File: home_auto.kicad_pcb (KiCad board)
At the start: 2 copper layers, 162 parts, among them J1 Conn_01x08_Pin, J10 Screw_Terminal_01x02, J11 Screw_Terminal_01x02, J12 Screw_Terminal_01x02, J13 Screw_Terminal_01x02, J14 Screw_Terminal_01x02, J15 Screw_Terminal_01x02, J16 Screw_Terminal_01x02, J17 Screw_Terminal_01x02, J18 Screw_Terminal_01x02, J19 Screw_Terminal_01x02, J2 Screw_Terminal_01x02, J20 Screw_Terminal_01x02, J21 Screw_Terminal_01x02, J22 Screw_Terminal_01x02, J23 Screw_Terminal_01x02, J24 Screw_Terminal_01x02, J25 Screw_Terminal_01x02, J26 Conn_01x02_Pin, J27 Conn_01x04_Pin, J28 Conn_01x02_Pin, J29 TC0203620000G, J3 Screw_Terminal_01x02, J4 Conn_02x10_Top_Bottom, J5 Conn_02x10_Top_Bottom, J6 Screw_Terminal_01x02, J7 Screw_Terminal_01x02, J8 Screw_Terminal_01x02, J9 Screw_Terminal_01x02, K1 G5NB-1A4_DC5, K10 G5NB-1A4_DC5, K11 G5NB-1A4_DC5, K12 G5NB-1A4_DC5, K13 G5NB-1A4_DC5, K14 G5NB-1A4_DC5, K15 G5NB-1A4_DC5, K16 G5NB-1A4_DC5, K17 G5NB-1A4_DC5, K18 G5NB-1A4_DC5, K19 G5NB-1A4_DC5, K2 G5NB-1A4_DC5, K20 G5NB-1A4_DC5, K21 G5NB-1A4_DC5, K22 G5NB-1A4_DC5, K23 G5NB-1A4_DC5, K24 G5NB-1A4_DC5, K25 G5NB-1A4_DC5, K26 G5NB-1A4_DC5, K27 G5NB-1A4_DC5, K28 G5NB-1A4_DC5, K3 G5NB-1A4_DC5, K4 G5NB-1A4_DC5, K5 G5NB-1A4_DC5, K6 G5NB-1A4_DC5, K7 G5NB-1A4_DC5, K8 G5NB-1A4_DC5, K9 G5NB-1A4_DC5, Q1 BC849, Q10 BC849, Q11 BC849, Q12 BC849, Q13 BC849, Q14 BC849, Q15 BC849, Q16 BC849, Q17 BC849, Q18 BC849, Q19 BC849, Q2 BC849, Q20 BC849, Q21 BC849, Q22 BC849, Q23 BC849, Q24 BC849, Q25 BC849, Q26 BC849, Q27 BC849, Q28 BC849, Q3 BC849, Q4 BC849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

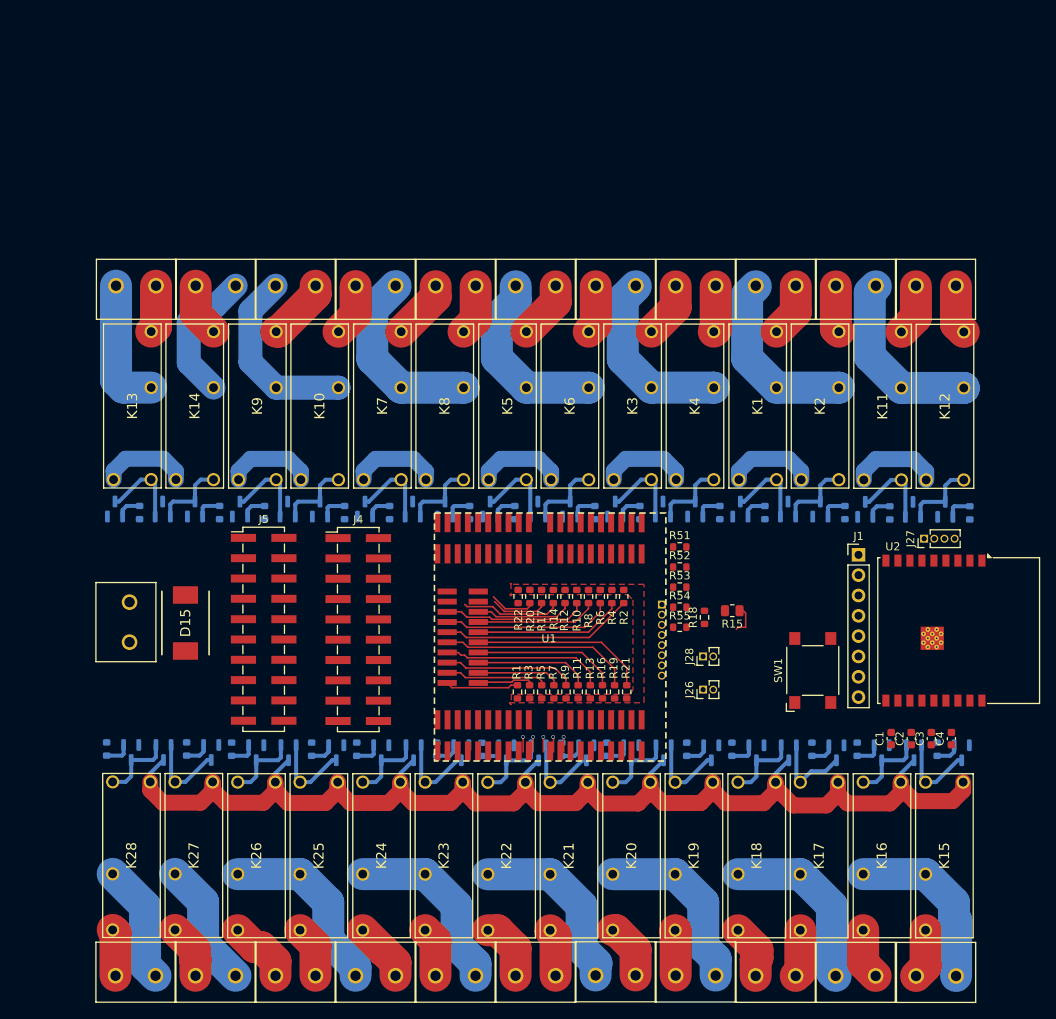
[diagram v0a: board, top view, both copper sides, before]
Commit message: filse fo JCL pcb generated
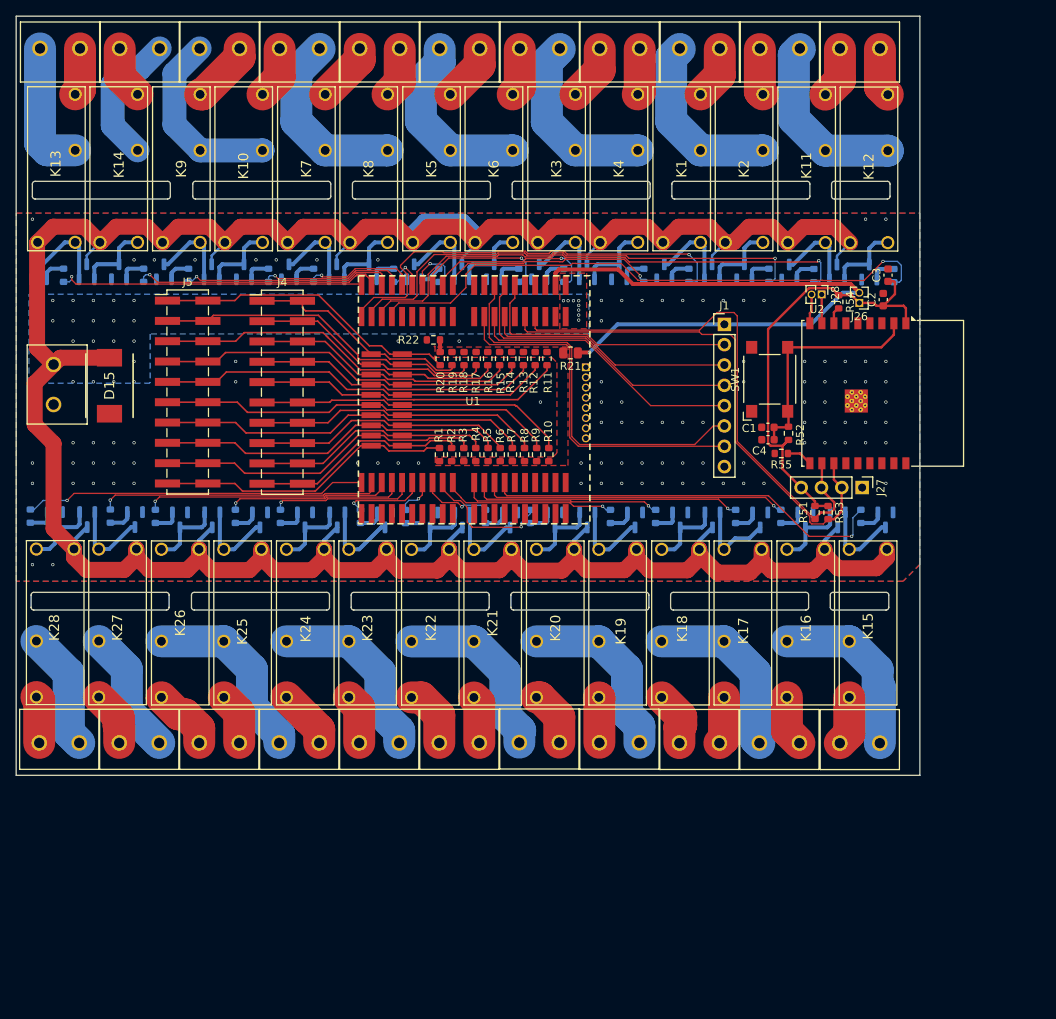
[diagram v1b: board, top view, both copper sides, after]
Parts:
- J27: footprint Connector_PinHeader_1.27mm:PinHeader_1x04_P1.27mm_Vertical -> Connector_PinHeader_2.54mm:PinHeader_1x04_P2.54mm_Vertical
- R15: value 0R -> 4K7; footprint Resistor_SMD:R_0805_2012Metric -> Resistor_SMD:R_0603_1608Metric
- R18: value 0R -> 4K7
- R21: value 4K7 -> 0R; footprint Resistor_SMD:R_0603_1608Metric -> Resistor_SMD:R_0805_2012Metric
- R22: value 4K7 -> 0R
- moved C3 58.2 mm to (250.6, 81.7)
- moved C2 55.0 mm to (250.0, 84.8)
- moved J26 52.1 mm to (247.0, 85.2), turned to 180 degrees
- moved J28 47.6 mm to (242.3, 84.1), turned to -90 degrees
- moved R19 46.3 mm to (196.1, 92.1), turned to 90 degrees
- moved R18 44.2 mm to (197.6, 92.1)
- moved R16 44.1 mm to (200.5, 92.1), turned to 90 degrees
- moved C4 43.8 mm to (235.6, 102.3), turned to 180 degrees
- moved R54 43.0 mm to (244.4, 85.0), turned to -90 degrees
- moved R21 42.9 mm to (210.9, 91.4), turned to 180 degrees
- moved R15 42.9 mm to (202.0, 92.1), turned to 90 degrees
- moved R13 42.5 mm to (205.0, 92.1), turned to 90 degrees
- moved C1 41.9 mm to (235.6, 100.7), turned to 180 degrees
- moved R11 41.8 mm to (207.9, 92.1), turned to 90 degrees
- moved SW1 36.8 mm to (235.8, 94.7)
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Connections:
- J4 pad 1: /sw_13 -> /sw_18
- J4 pad 10: /sw_14 -> /sw_10
- J4 pad 11: /sw_15 -> /sw_9
- J4 pad 12: /sw_15 -> /sw_9
- J4 pad 13: /sw_16 -> /sw_7
- J4 pad 14: /sw_16 -> /sw_7
- J4 pad 15: /sw_17 -> /sw_5
- J4 pad 16: /sw_17 -> /sw_5
- J4 pad 17: /sw_18 -> /sw_3
- J4 pad 18: /sw_18 -> /sw_3
- J4 pad 19: /sw_19 -> /sw_1
- J4 pad 2: /sw_13 -> /sw_18
- J4 pad 20: /sw_19 -> /sw_1
- J4 pad 3: /sw_12 -> /sw_16
- J4 pad 4: /sw_12 -> /sw_16
- J4 pad 5: /sw_11 -> /sw_14
- J4 pad 6: /sw_11 -> /sw_14
- J4 pad 7: /sw_10 -> /sw_12
- J4 pad 8: /sw_10 -> /sw_12
- J4 pad 9: /sw_14 -> /sw_10
- J5 pad 1: /sw_3 -> /sw_19
- J5 pad 10: /sw_4 -> /sw_11
- J5 pad 11: /sw_5 -> /sw_8
- J5 pad 12: /sw_5 -> /sw_8
- J5 pad 15: /sw_7 -> /sw_4
- J5 pad 16: /sw_7 -> /sw_4
- J5 pad 17: /sw_8 -> /sw_2
- J5 pad 18: /sw_8 -> /sw_2
- J5 pad 19: /sw_9 -> /sw_0
- J5 pad 2: /sw_3 -> /sw_19
- J5 pad 20: /sw_9 -> /sw_0
- J5 pad 3: /sw_2 -> /sw_17
- J5 pad 4: /sw_2 -> /sw_17
- J5 pad 5: /sw_1 -> /sw_15
- J5 pad 6: /sw_1 -> /sw_15
- J5 pad 7: /sw_0 -> /sw_13
- J5 pad 8: /sw_0 -> /sw_13
- J5 pad 9: /sw_4 -> /sw_11
- R1 pad 1: /sw_10 -> /sw_0
- R10 pad 1: /sw_4 -> /sw_9
- R11 pad 1: /sw_15 -> /sw_10
- R12 pad 1: /sw_5 -> /sw_11
- R13 pad 1: /sw_16 -> /sw_12
- R14 pad 1: /sw_6 -> /sw_13
- R15 pad 1: +3V3 -> /sw_14
- R16 pad 1: /sw_17 -> /sw_15
- R17 pad 1: /sw_7 -> /sw_16
- R18 pad 1: GND -> /sw_17
- R2 pad 1: /sw_0 -> /sw_1
- R20 pad 1: /sw_8 -> /sw_19
- R21 pad 1: /sw_19 -> +3V3
- R22 pad 1: /sw_9 -> GND
- R23 pad 2: /led_cur_lim2/UP -> /up_2
- R24 pad 2: /led_cur_lim2/DOWN -> /down_2
- R25 pad 2: /led_cur_lim3/UP -> /up_3
- R26 pad 2: /led_cur_lim3/DOWN -> /down_3
- R27 pad 2: /led_cur_lim4/UP -> /up_4
- R28 pad 2: /led_cur_lim4/DOWN -> /down_4
- R29 pad 2: /led_cur_lim5/UP -> /up_5
- R3 pad 1: /sw_11 -> /sw_2
- R30 pad 2: /led_cur_lim5/DOWN -> /down_5
- R31 pad 2: /led_cur_lim6/UP -> /up_6
- R32 pad 2: /led_cur_lim6/DOWN -> /down_6
- R33 pad 2: /led_cur_lim1/UP -> /up_1
- R34 pad 2: /led_cur_lim1/DOWN -> /down_1
- R35 pad 2: /led_cur_lim7/UP -> /up_7
- R36 pad 2: /led_cur_lim7/DOWN -> /down_7
- R37 pad 2: /led_cur_lim8/UP -> /up_8
- R38 pad 2: /led_cur_lim8/DOWN -> /down_8
- R39 pad 2: /led_cur_lim9/UP -> /up_9
- R4 pad 1: /sw_1 -> /sw_3
- R40 pad 2: /led_cur_lim9/DOWN -> /down_9
- R41 pad 2: /led_cur_lim10/UP -> /up_A
- R42 pad 2: /led_cur_lim10/DOWN -> /down_A
- R43 pad 2: /led_cur_lim11/UP -> /up_B
- R44 pad 2: /led_cur_lim11/DOWN -> /down_B
- R45 pad 2: /led_cur_lim12/UP -> /up_C
- R46 pad 2: /led_cur_lim12/DOWN -> /down_C
- R47 pad 2: /led_cur_lim13/UP -> /up_D
- R48 pad 2: /led_cur_lim13/DOWN -> /down_D
- R49 pad 2: /led_cur_lim14/UP -> /up_E
- R5 pad 1: /sw_12 -> /sw_4
- R50 pad 2: /led_cur_lim14/DOWN -> /down_E
- R6 pad 1: /sw_2 -> /sw_5
- R7 pad 1: /sw_13 -> /sw_6
- R8 pad 1: /sw_3 -> /sw_7
- R9 pad 1: /sw_14 -> /sw_8
- U1 pad B11: /RX -> /TX
- U1 pad B13: /TX -> /RX
- U1 pad C0: /UP_12 -> /up_7
- U1 pad C1: unconnected-(U1B-GPIO15-PadC1) -> /up_2
- U1 pad C10: /DOWN_14 -> /down_5
- U1 pad C12: /UP_14 -> /up_4
- U1 pad C14: /DOWN_13 -> /down_4
- U1 pad C16: /UP_13 -> /up_3
- U1 pad C18: /DOWN_12 -> /down_3
- U1 pad C2: /DOWN_11 -> /down_7
- U1 pad C3: unconnected-(U1B-GPIO17-PadC3) -> /down_2
- U1 pad C4: /UP_11 -> /up_6
- U1 pad C5: unconnected-(U1B-GPIO19-PadC5) -> /up_1
- U1 pad C6: /DOWN_10 -> /down_6
- U1 pad C7: unconnected-(U1B-GPIO21-PadC7) -> /down_1
- U1 pad C8: /UP_10 -> /up_5
- U1 pad D0: /sw_10 -> /sw_0
- U1 pad D1: /sw_11 -> /sw_1
- U1 pad D10: /sw_0 -> /sw_10
- U1 pad D11: /sw_1 -> /sw_11
- U1 pad D12: /sw_2 -> /sw_12
- U1 pad D13: /sw_3 -> /sw_13
- U1 pad D14: /sw_4 -> /sw_14
- U1 pad D15: /sw_5 -> /sw_15
- U1 pad D16: /sw_6 -> /sw_16
- U1 pad D17: /sw_7 -> /sw_17
- U1 pad D18: /sw_8 -> /sw_18
- U1 pad D19: /sw_9 -> /sw_19
- U1 pad D2: /sw_12 -> /sw_2
- U1 pad D3: /sw_13 -> /sw_3
- U1 pad D4: /sw_14 -> /sw_4
- U1 pad D5: /sw_15 -> /sw_5
- U1 pad D6: /sw_16 -> /sw_6
- U1 pad D7: /sw_17 -> /sw_7
- U1 pad D8: /sw_18 -> /sw_8
- U1 pad D9: /sw_19 -> /sw_9
- U1 pad E0: unconnected-(U1D-GPIO54-PadE0) -> /down_E
- U1 pad E10: unconnected-(U1D-DIF_0_p-PadE10) -> /up_C
- U1 pad E12: unconnected-(U1D-DIF_0_n-PadE12) -> /down_B
- U1 pad E14: unconnected-(U1D-DIF_2_p-PadE14) -> /up_B
- U1 pad E16: unconnected-(U1D-DIF_2_n-PadE16) -> /down_A
- U1 pad E18: unconnected-(U1D-DIF_4_p-PadE18) -> /up_A
- U1 pad E2: unconnected-(U1D-GPIO56-PadE2) -> /up_E
- U1 pad E4: unconnected-(U1D-GPIO58-PadE4) -> /down_D
- U1 pad E6: unconnected-(U1D-GPIO60-PadE6) -> /up_D
- U1 pad E8: unconnected-(U1D-GPIO62-PadE8) -> /down_C
- U1 pad F0: unconnected-(U1E-DIF_4_n-PadF0) -> /down_9
- U1 pad F2: unconnected-(U1E-DIF_6_p-PadF2) -> /up_9
- U1 pad F4: unconnected-(U1E-DIF_6_n-PadF4) -> /down_8
- U1 pad F6: unconnected-(U1E-DIF_8_p-PadF6) -> /up_8
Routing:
- net +5V: track 247.3 -> 376.1 mm, vias 0 -> 8
- net +3V3: track 3.93 -> 79.2 mm, vias 0 -> 1
- net /down_1: track 0.00 -> 72.9 mm, vias 0 -> 1
- net /RX: track 0.00 -> 66.7 mm
- net /TX: track 0.00 -> 66.3 mm
- net /up_1: track 0.00 -> 64.0 mm, vias 0 -> 1
- net /down_2: track 0.00 -> 60.0 mm, vias 0 -> 1
- net +3V3_ESP: track 0.00 -> 55.9 mm
- net /up_2: track 0.00 -> 53.6 mm, vias 0 -> 1
- net /up_8: track 0.00 -> 50.8 mm, vias 0 -> 1
- net /mux_5: track 0.00 -> 49.2 mm
- net /mux_4: track 0.00 -> 45.0 mm
- net /sw_8: track 5.91 -> 49.8 mm
- net /down_E: track 0.00 -> 42.8 mm, vias 0 -> 1
- net /sw_11: track 7.08 -> 49.6 mm
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- added copper zone on B.Cu, net +5V
- added copper zone on F.Cu, net +5V
- added copper zone on B.Cu, net GND
- added copper zone on F.Cu, net GND
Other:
- board outline added: 113 x 94.9 mm
